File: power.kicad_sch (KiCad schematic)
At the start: 16 parts, among them J2 USB_C_Receptacle_PowerOnly_6P

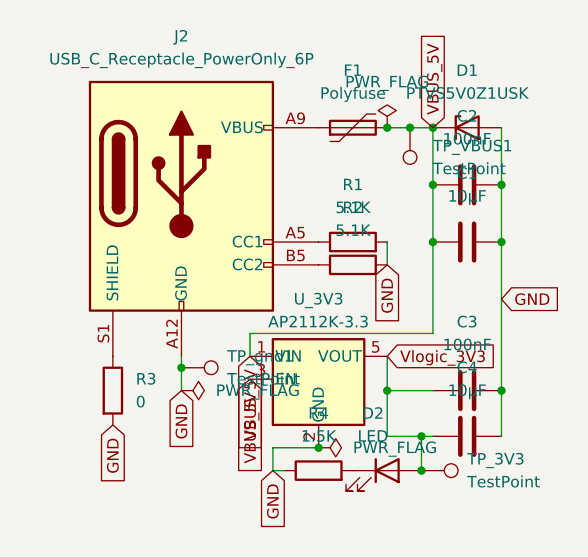
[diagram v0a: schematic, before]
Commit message: Add files via upload
V4 : full and final v1.1. Working schematics. Working PCB layout, zero ERC and DRC errors and warnings(except for cosmetic ones).
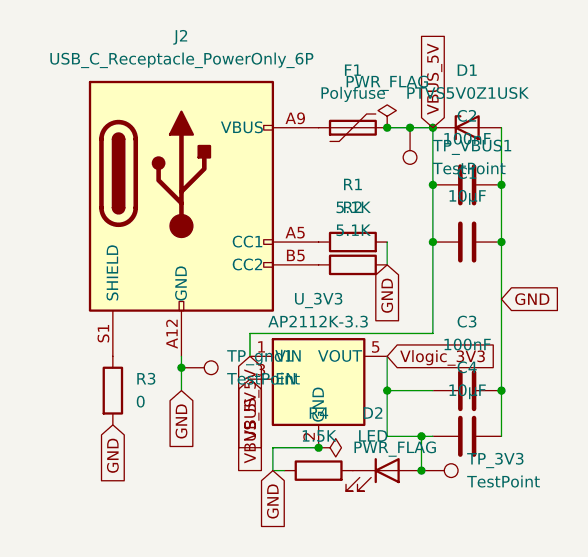
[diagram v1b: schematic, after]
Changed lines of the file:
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@@
-	)
-	(symbol
-		(lib_id "power:PWR_FLAG")
-		(at 120.65 60.96 270)
-		(unit 1)
-		(exclude_from_sim no)
-		(in_bom yes)
-		(on_board yes)
-		(dnp no)
-		(fields_autoplaced yes)
-		(property "Reference" "#FLG02"
-			(at 122.555 60.96 0)
-			(effects
-				(font
-					(size 1.27 1.27)
-				)
-				(hide yes)
-			)
-		)
-		(property "Value" "PWR_FLAG"
-			(at 124.46 60.9599 90)
-			(effects
-				(font
-					(size 1.27 1.27)
-				)
-				(justify left)
-			)
-		)
-		(property "Footprint" ""
-			(at 120.65 60.96 0)
-			(effects
-				(font
-					(size 1.27 1.27)
-				)
-				(hide yes)
-			)
-		)
-		(property "Datasheet" "~"
-			(at 120.65 60.96 0)
-			(effects
-				(font
-					(size 1.27 1.27)
-				)
-				(hide yes)
-			)
-		)
-		(property "Description" "Special symbol for telling ERC where power comes from"
-			(at 120.65 60.96 0)
-			(effects
-				(font
-					(size 1.27 1.27)
-				)
-				(hide yes)
-			)
-		)
-		(pin "1"
-		)
-		(instances
-			(project ""
-				(path "/c8d0e3cf-b697-430c-b4f3-c5285558b4ca/a3d1f251-0cce-4493-9b12-767abad6ca7c"
-					(reference "#FLG02")
-					(unit 1)
-				)
-			)
-		)
 	)
 	(symbol

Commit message: Add files via upload
V5 : complete finish for v1, directly to-the-fab design.
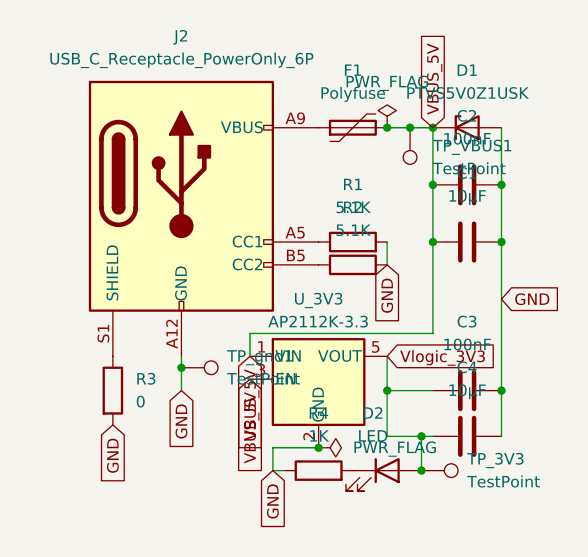
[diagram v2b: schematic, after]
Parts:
- C1, C4: LCSC (none) -> C15850
- C2, C3: LCSC (none) -> C49678
- D1: LCSC (none) -> C85364
- D2: LCSC (none) -> C2827270
- F1: LCSC (none) -> C70059
- J2: LCSC (none) -> C283540
- R1, R2: LCSC (none) -> C23186
- R3: LCSC (none) -> C17477
- R4: value 1.5K -> 1K; LCSC (none) -> C17604
- TP_3V3, TP_VBUS1, TP_gnd1: now left out of the parts list
- U_3V3: LCSC (none) -> C51118
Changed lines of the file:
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@@
+			)
+		)
+		(property "LCSC" "C85364"
+			(at 152.4 31.75 0)
+			(effects
+				(font
+					(size 1.27 1.27)
+				)
+				(hide yes)
 			)
 		)
@@
 			)
 		)
+		(property "LCSC" "C15850"
+			(at 152.4 66.04 90)
+			(effects
+				(font
+					(size 1.27 1.27)
+				)
+				(hide yes)
+			)
+		)
 		(pin "1"
 		)
@@
 			)
 		)
-		(property "Value" "1.5K"
+		(property "Value" "1K"
 			(at 135.89 66.04 90)
 			(effects
@@
 			)
 		)
+		(property "LCSC" "C17604"
+			(at 135.89 69.85 90)
+			(effects
+				(font
+					(size 1.27 1.27)
+				)
+				(hide yes)
+			)
+		)
 		(pin "1"
 		)
@@
 			)
 		)
+		(property "LCSC" "C51118"
+			(at 135.89 59.69 0)
+			(effects
+				(font
+					(size 1.27 1.27)
+				)
+				(hide yes)
+			)
+		)
 		(pin "1"
 		)
@@
 		(unit 1)
 		(exclude_from_sim no)
-		(in_bom yes)
+		(in_bom no)
 		(on_board yes)
 		(dnp no)
@@
 			)
 		)
+		(property "LCSC" ""
+			(at 146.05 31.75 0)
+			(effects
+				(font
+					(size 1.27 1.27)
+				)
+				(hide yes)
+			)
+		)
 		(pin "1"
 		)
@@
 			)
 		)
+		(property "LCSC" "C17477"
+			(at 113.03 60.96 0)
+			(effects
+				(font
+					(size 1.27 1.27)
+				)
+				(hide yes)
+			)
+		)
 		(pin "2"
 		)
@@
 			)
 		)
+		(property "LCSC" "C23186"
+			(at 139.7 44.45 90)
+			(effects
+				(font
+					(size 1.27 1.27)
+				)
+				(hide yes)
+			)
+		)
 		(pin "2"
 		)
@@
 			)
 		)
+		(property "LCSC" "C49678"
+			(at 152.4 60.96 90)
+			(effects
+				(font
+					(size 1.27 1.27)
+				)
+				(hide yes)
+			)
+		)
 		(pin "1"
 		)
@@
 			)
 		)
+		(property "LCSC" "C49678"
+			(at 152.4 38.1 90)
+			(effects
+				(font
+					(size 1.27 1.27)
+				)
+				(hide yes)
+			)
+		)
 		(pin "2"
 		)
@@
 			)
 		)
+		(property "LCSC" "C283540"
+			(at 120.65 39.37 0)
+			(effects
+				(font
+					(size 1.27 1.27)
+				)
+				(hide yes)
+			)
+		)
 		(pin "B12"
 		)
@@
 			)
 		)
+		(property "LCSC" "C15850"
+			(at 152.4 44.45 90)
+			(effects
+				(font
+					(size 1.27 1.27)
+				)
+				(hide yes)
+			)
+		)
 		(pin "1"
 		)
@@
 			)
 		)
+		(property "LCSC" "C23186"
+			(at 139.7 46.99 90)
+			(effects
+				(font
+					(size 1.27 1.27)
+				)
+				(hide yes)
+			)
+		)
 		(pin "2"
 		)
@@
 			)
 		)
+		(property "LCSC" "C2827270"
+			(at 143.51 69.85 0)
+			(effects
+				(font
+					(size 1.27 1.27)
+				)
+				(hide yes)
+			)
+		)
 		(pin "2"
 		)
@@
 			)
 		)
+		(property "LCSC" "C70059"
+			(at 139.7 31.75 90)
+			(effects
+				(font
+					(size 1.27 1.27)
+				)
+				(hide yes)
+			)
+		)
 		(pin "1"
 		)
@@
 		(unit 1)
 		(exclude_from_sim no)
-		(in_bom yes)
+		(in_bom no)
 		(on_board yes)
 		(dnp no)
@@
 			)
 		)
+		(property "LCSC" ""
+			(at 147.32 69.85 90)
+			(effects
+				(font
+					(size 1.27 1.27)
+				)
+				(hide yes)
+			)
+		)
 		(pin "1"
 		)
@@
 		(unit 1)
 		(exclude_from_sim no)
-		(in_bom yes)
+		(in_bom no)
 		(on_board yes)
 		(dnp no)
@@
 			(effects
 				(font
+					(size 1.27 1.27)
+				)
+				(hide yes)
+			)
+		)
+		(property "LCSC" ""
+			(at 120.65 58.42 90)
+			(effects
+				(font
